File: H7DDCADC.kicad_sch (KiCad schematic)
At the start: 21 parts, among them J1 U.FL-DNP, J2 SMA, J3 SMA, J4 HDR2, U1 74AUC1G74DCT, U2 74AUC1G74DCT

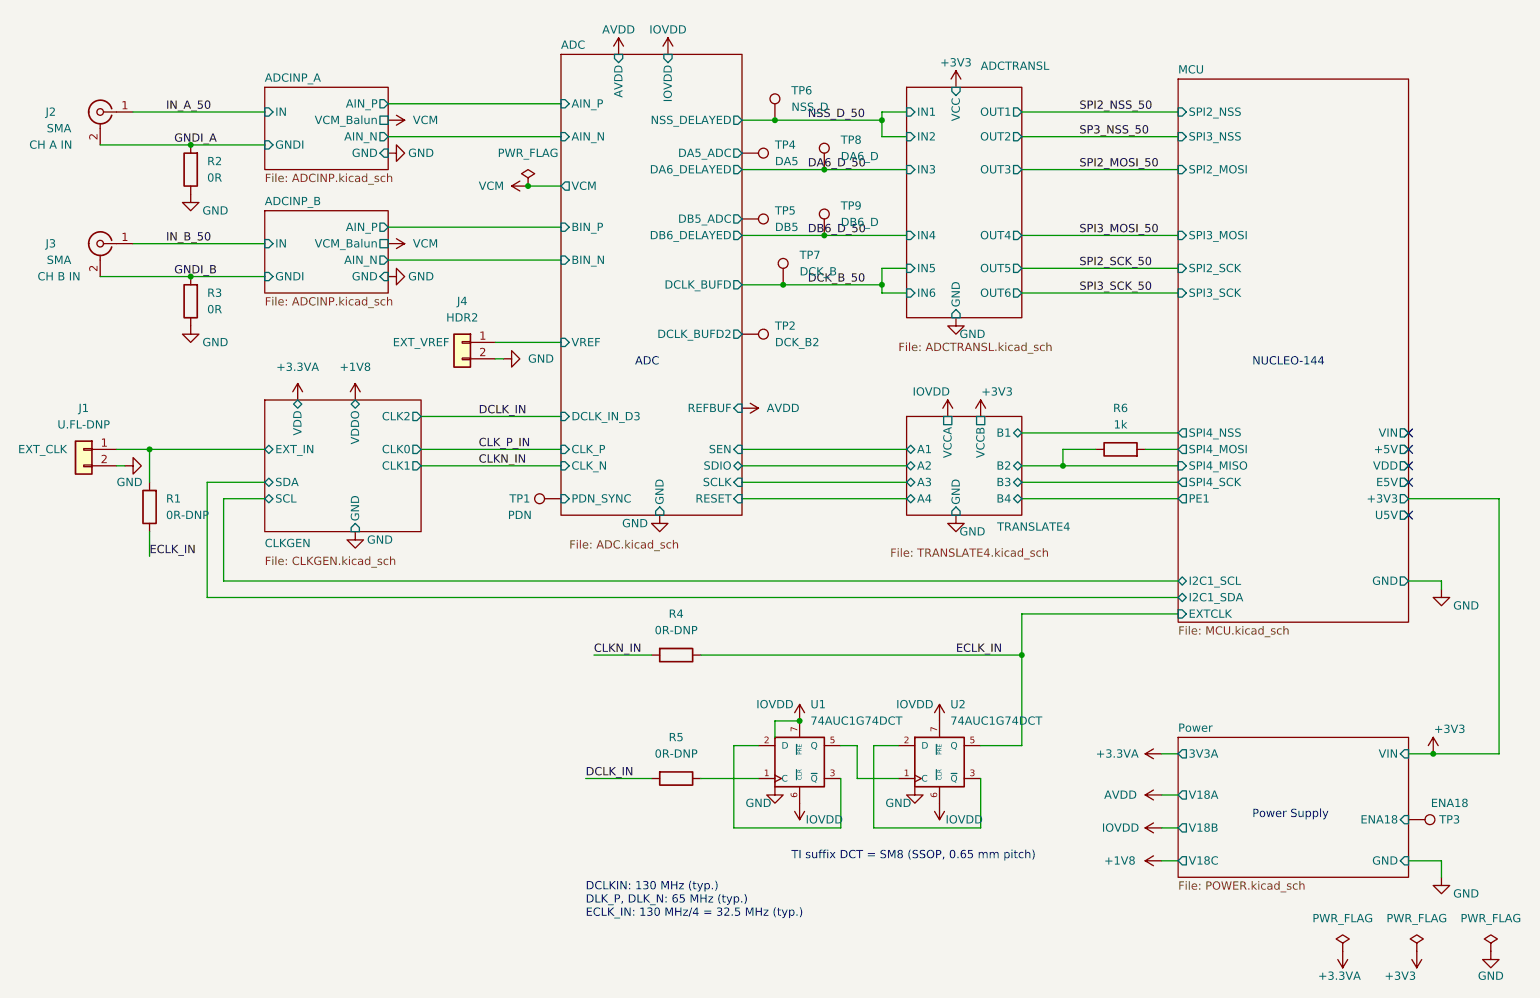
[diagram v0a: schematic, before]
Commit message: routing in progress 1
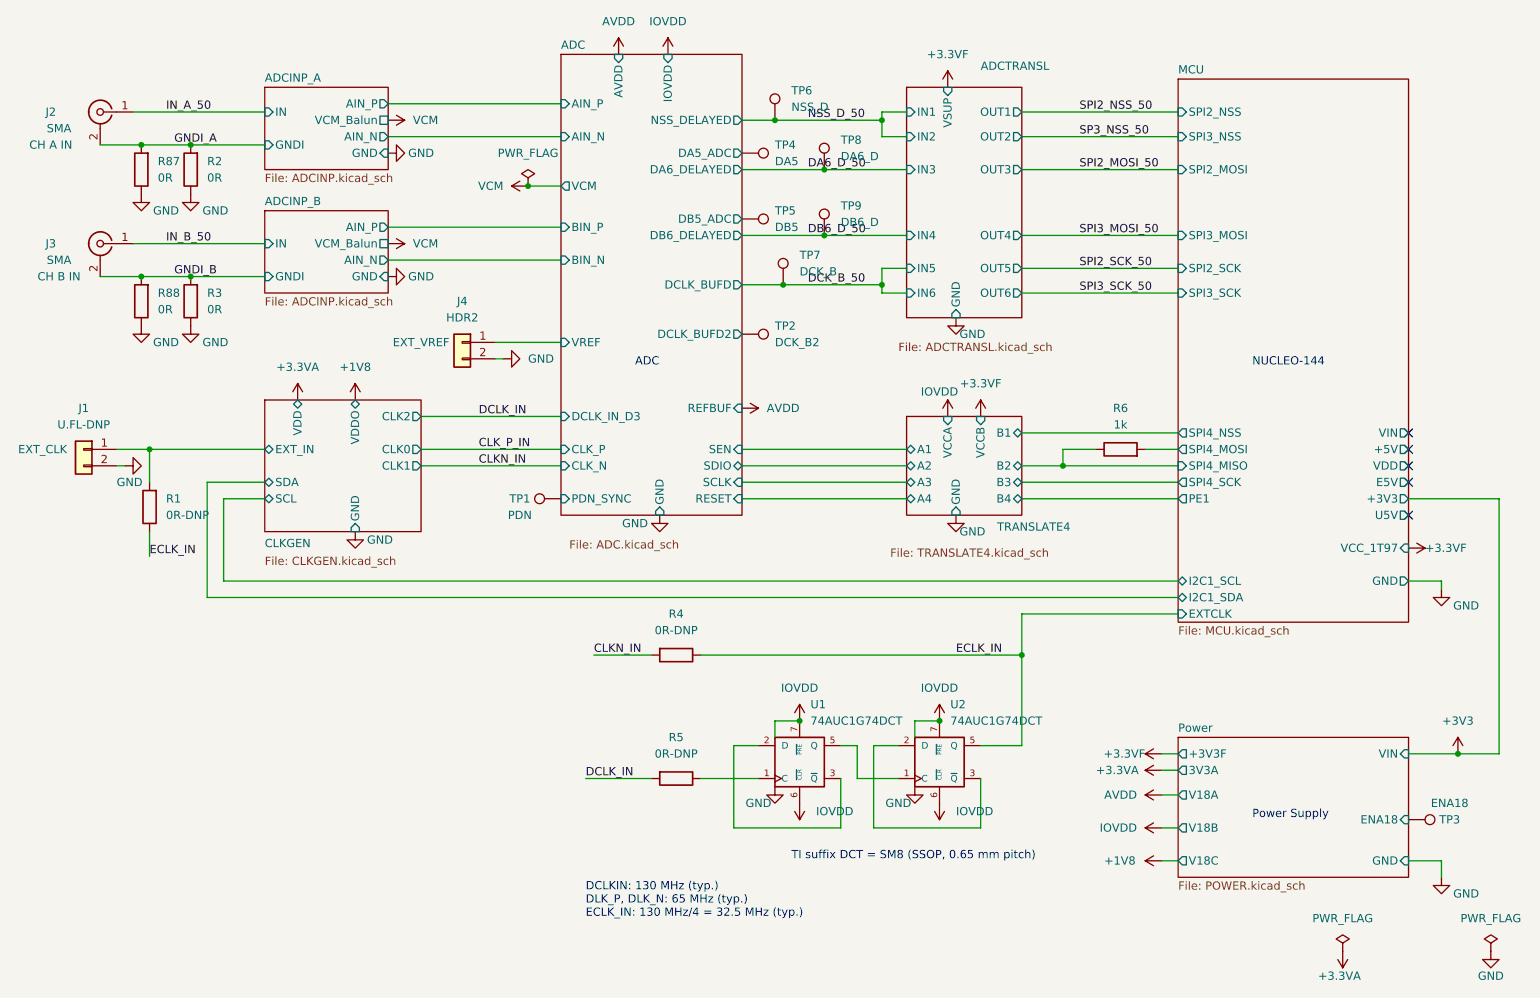
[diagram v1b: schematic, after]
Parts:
- added R87, R88: 0R, Resistor_SMD:R_0805_2012Metric, symbol Device:R
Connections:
- net GND: now also R87.1, R88.1
- net GNDI_A: now also R87.2
- net GNDI_B: now also R88.2
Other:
- sheet ADCTRANSL ports: added VSUP; removed VCC
- sheet MCU ports: added VCC_1T97; removed none
- sheet Power ports: added +3V3F; removed none
